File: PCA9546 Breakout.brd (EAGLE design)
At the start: 17.8 x 20.3 mm, 21 parts, among them U2 PCA9546A TSSOP

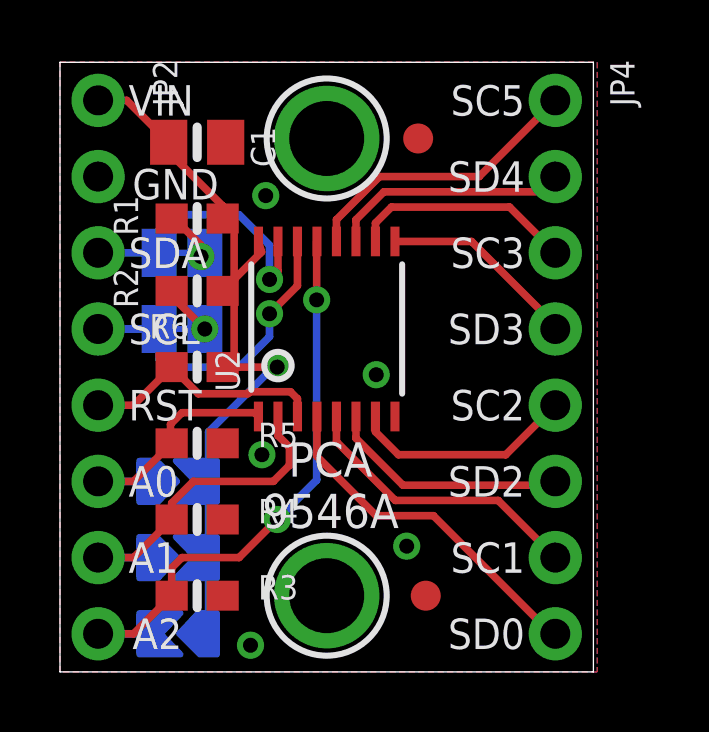
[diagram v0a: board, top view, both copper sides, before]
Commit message: new silk
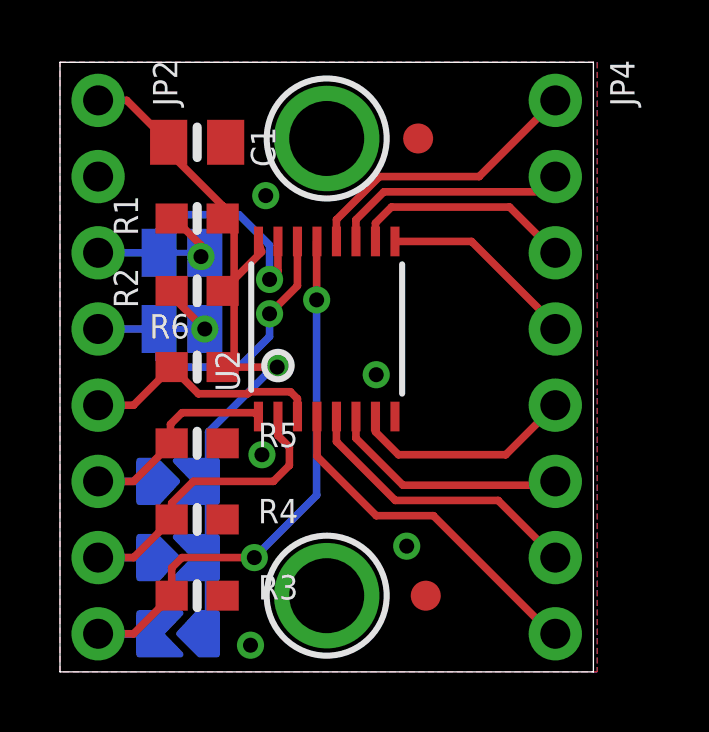
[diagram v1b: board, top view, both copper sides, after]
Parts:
- added PLABEL0: (no value), pinguin:PLABEL0
- added PLABEL1: (no value), pinguin:PLABEL1
- added PLABEL10: (no value), pinguin:PLABEL10
- added PLABEL11: (no value), pinguin:PLABEL11
- added PLABEL12: (no value), pinguin:PLABEL12
- added PLABEL13: (no value), pinguin:PLABEL13
- added PLABEL14: (no value), pinguin:PLABEL14
- added PLABEL15: (no value), pinguin:PLABEL15
- added PLABEL16: (no value), pinguin:PLABEL16
- added PLABEL17: (no value), pinguin:PLABEL17
- added PLABEL18: (no value), pinguin:PLABEL18
- added PLABEL19: (no value), pinguin:PLABEL19
- added PLABEL2: (no value), pinguin:PLABEL2
- added PLABEL20: (no value), pinguin:PLABEL20
- added PLABEL21: (no value), pinguin:PLABEL21
- added PLABEL22: (no value), pinguin:PLABEL22
- added PLABEL3: (no value), pinguin:PLABEL3
- added PLABEL4: (no value), pinguin:PLABEL4
- added PLABEL5: (no value), pinguin:PLABEL5
- added PLABEL6: (no value), pinguin:PLABEL6
- added PLABEL7: (no value), pinguin:PLABEL7
- added PLABEL8: (no value), pinguin:PLABEL8
- added PLABEL9: (no value), pinguin:PLABEL9
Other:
- board text added: "SC0"
- board text added: "SD1"
- board text removed: "SC5"
- board text removed: "SD4"
